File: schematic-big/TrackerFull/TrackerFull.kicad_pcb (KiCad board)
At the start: 2 copper layers, 43.2 x 46.9 mm, 61 parts, among them J1 Conn_01x02_Male, J2 Conn_01x02_Male, J3 Screw_Terminal_01x02, J4 78646-3001, J5 Screw_Terminal_01x02, Q1 IRLML0030, Q2 IRLML5203, Q3 IRLML5203, SW1 SW_Push, U1 LP2985-3.3, U2 LIS3DSH, U3 ATtiny85-20PU, U4 MCP73831-2-OT, U5 U.FL

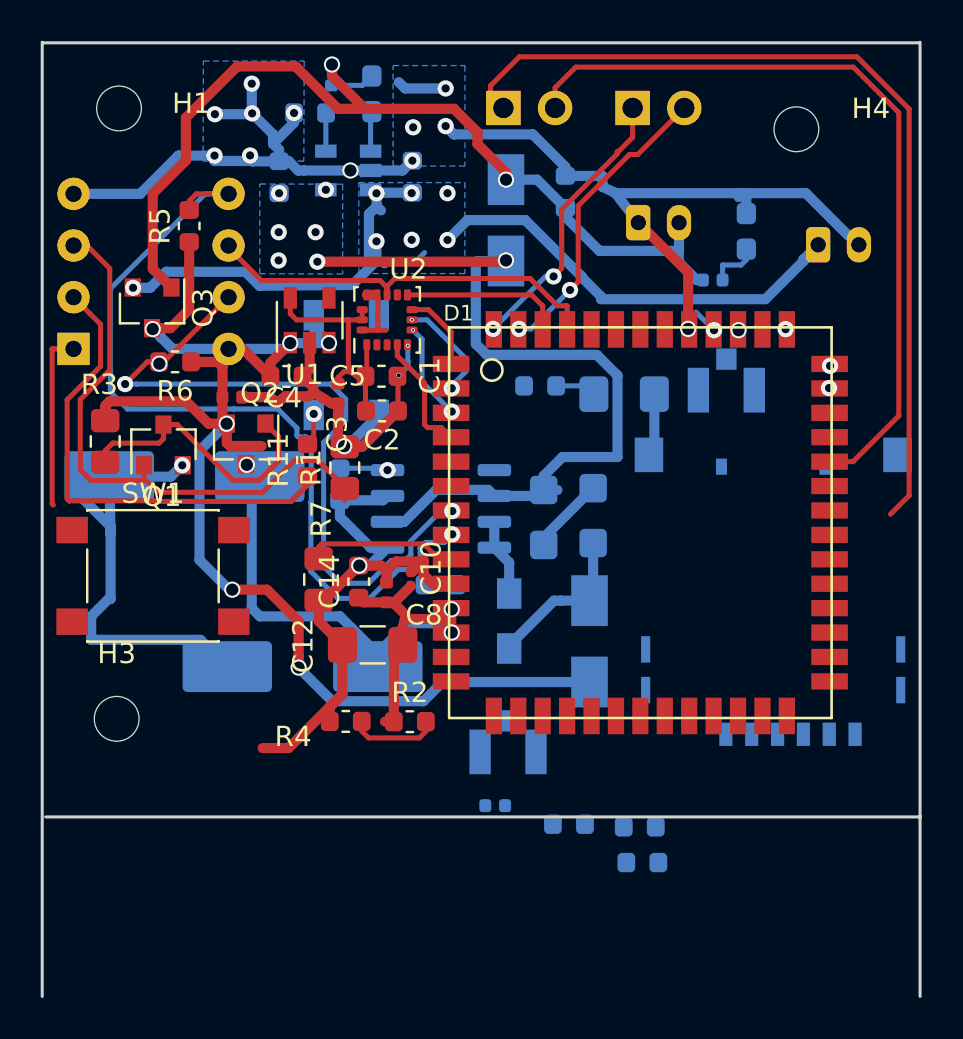
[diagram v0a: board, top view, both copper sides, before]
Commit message: last changes
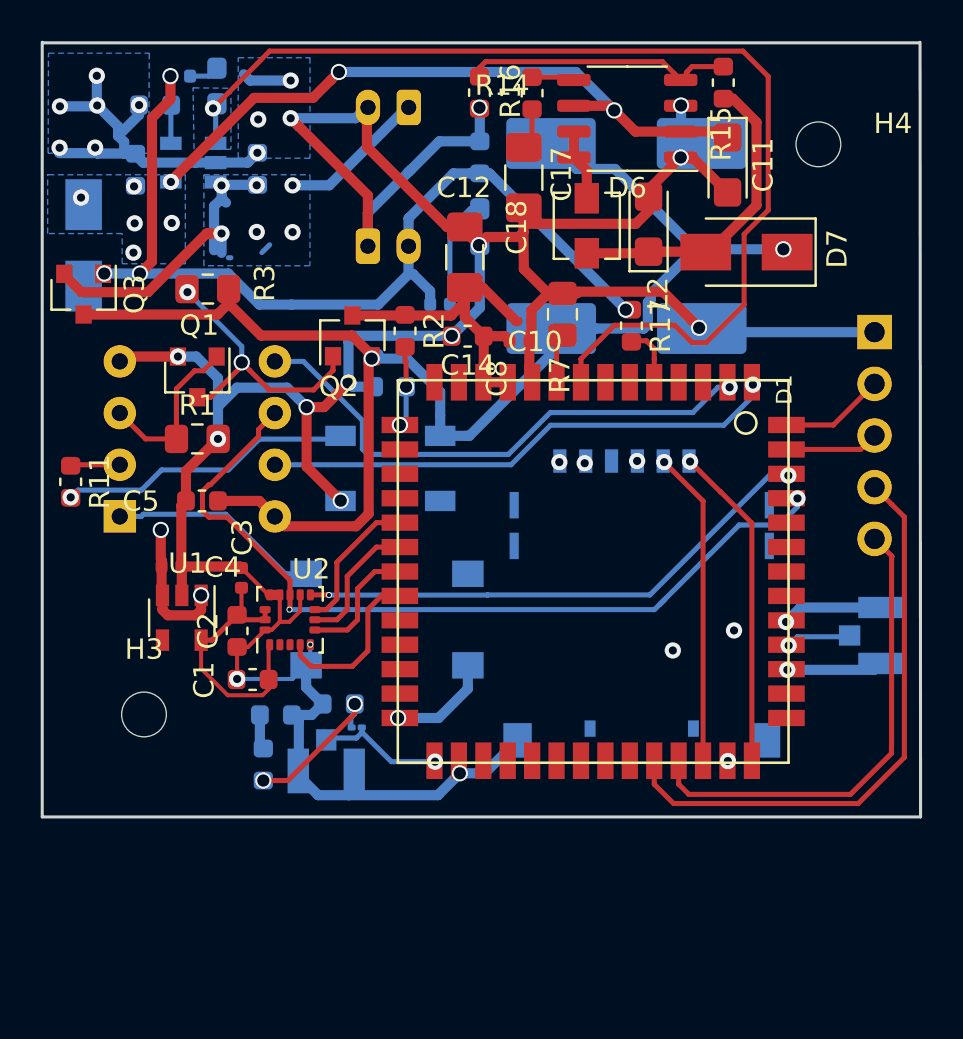
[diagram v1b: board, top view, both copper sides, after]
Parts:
- removed H1: MountingHole, MountingHole:MountingHole_2.2mm_M2
- removed J2: Conn_01x02_Male, Connector_PinHeader_2.54mm:PinHeader_1x02_P2.54mm_Vertical
- removed R5, R6: 10K, Resistor_SMD:R_0603_1608Metric
- added R17: 10K, Resistor_SMD:R_0603_1608Metric, F.Cu at (192.8, 80.3)
- C11, C17, C18, D6, D7, L2, R14, R15, R16: moved to F.Cu
- J1: value Conn_01x02_Male -> Conn_01x05_Male; footprint Connector_PinHeader_2.54mm:PinHeader_1x02_P2.54mm_Vertical -> Connector_PinHeader_2.54mm:PinHeader_1x05_P2.54mm_Vertical
- L1: footprint Inductor_SMD:L_0402_1005Metric -> Inductor_SMD:L_01005_0402Metric
- R4, SW1: moved to B.Cu
- moved R15 28.3 mm to (197.4, 68.4), turned to 90 degrees
- moved C15 27.2 mm to (192.6, 71.4), turned to 0 degrees
- moved C16 23.0 mm to (192.6, 80.5), turned to 0 degrees
- moved J1 21.3 mm to (204.8, 80.6), turned to 180 degrees
- moved D6 21.3 mm to (192.6, 70.1), turned to 180 degrees
- moved J3 21.2 mm to (181.9, 69.6), turned to 180 degrees
- moved D3 20.8 mm to (165.9, 76.4), turned to 270 degrees
- moved D7 20.6 mm to (198.5, 76.7), turned to 180 degrees
- moved R16 20.4 mm to (185.4, 68.9)
- moved L2 19.8 mm to (190.6, 75.4)
- moved C12 19.6 mm to (184.7, 77.0), turned to 90 degrees
- moved C11 19.5 mm to (197.6, 72.4)
- moved R2 19.2 mm to (181.7, 80.6), turned to 270 degrees
- moved R13 18.8 mm to (174.8, 101.9), turned to 270 degrees
- moved R7 17.7 mm to (189.5, 79.8), turned to 270 degrees
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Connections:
- C15 pad 1: /VBAT -> BAT_IN
- C16 pad 1: /VBAT -> BAT_IN
- D1 pad 1: /ACCEL_CS -> /AVR_SCK
- D1 pad 19: (no net) -> /ACCEL_CS
- D1 pad 2: /ACCEL_SDO -> /AVR_MOSI_SDA
- D1 pad 20: (no net) -> /ACCEL_SDO
- D1 pad 21: (no net) -> /ACCEL_SDA
- D1 pad 22: (no net) -> /ACCEL_SCL
- D1 pad 3: /ACCEL_SDA -> (no net)
- D1 pad 4: /ACCEL_SCL -> (no net)
- D1 pad 5: (no net) -> Net-(D1-Pad5)
- D1 pad 7: /AVR_SCK -> (no net)
- D1 pad 8: /AVR_MOSI_SDA -> /CHARGER_STAT
- J1 pad 1: /HST_RXD -> GNDREF
- J1 pad 2: /HST_TXD -> /UART1_TXD
- L1 pad 1: (no net) -> Net-(C13-Pad1)
- L1 pad 2: (no net) -> /GPS_RF
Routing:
- net GNDREF: track 142.5 -> 195.4 mm, vias 18 -> 28
- net /CHARGER_STAT: track 1.97 -> 53.6 mm, vias 0 -> 1
- net /ACCEL_INT1: track 19.9 -> 41.3 mm, vias 0 -> 2
- net Net-(R11-Pad1): track 23.9 -> 2.54 mm
- net /PWR_CTRL: track 29.0 -> 8.43 mm
- net /HST_RXD: track 44.0 -> 23.6 mm
- net /V_BAT: track 42.2 -> 23.9 mm, vias 7 -> 6
- net /ACCEL_INT2: track 8.02 -> 25.9 mm, vias 0 -> 2
- net /SIM_CLK: track 0.00 -> 16.0 mm
- net /SIM_IO: track 0.00 -> 15.5 mm, vias 0 -> 1
- net /AVR_MOSI_SDA: track 41.9 -> 26.4 mm
- net /VBAT: track 32.6 -> 19.1 mm, vias 3 -> 0
- net /LED_CTL: track 1.61 -> 14.5 mm
- net Net-(D6-Pad4): track 2.38 -> 13.7 mm, vias 1 -> 0
- net /UART1_RXD: track 14.8 -> 4.77 mm, vias 2 -> 0
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- added copper zone on B.Cu, net /CHARGER_STAT
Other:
- board size 43.2 x 46.9 mm -> 43.2 x 38.1 mm
